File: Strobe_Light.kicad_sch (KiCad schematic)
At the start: 15 parts, among them J4 ErrorLightConn, Q1 NTR4003NT1G, Q2 VND5N07-E, U1 SI8261ABC-IS

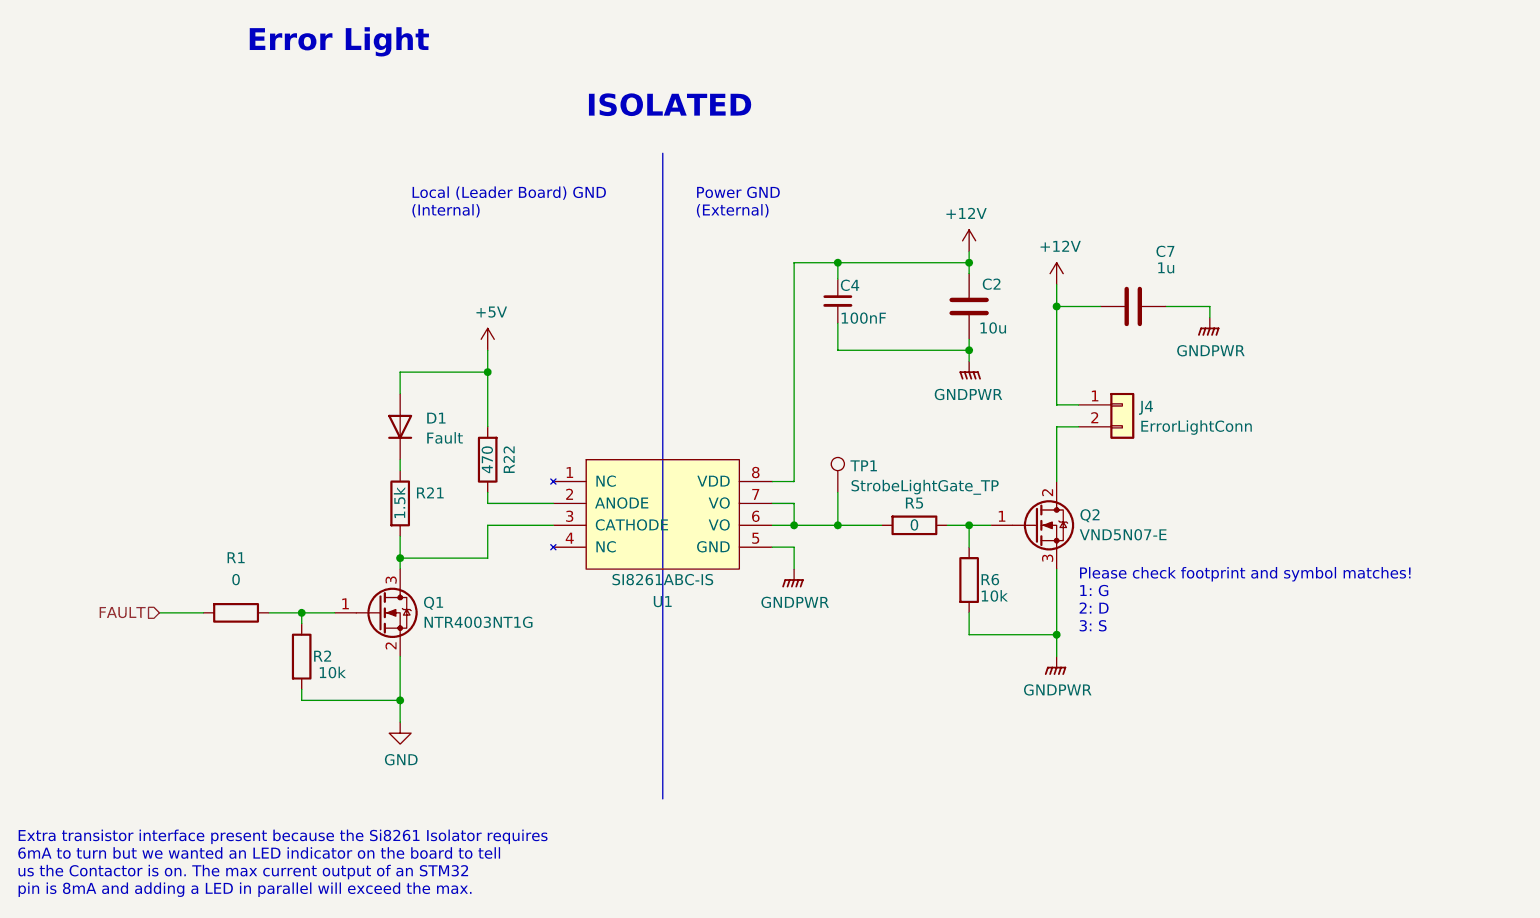
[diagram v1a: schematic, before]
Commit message: Finished comments for Strobe Light and started resolving them for Contactor
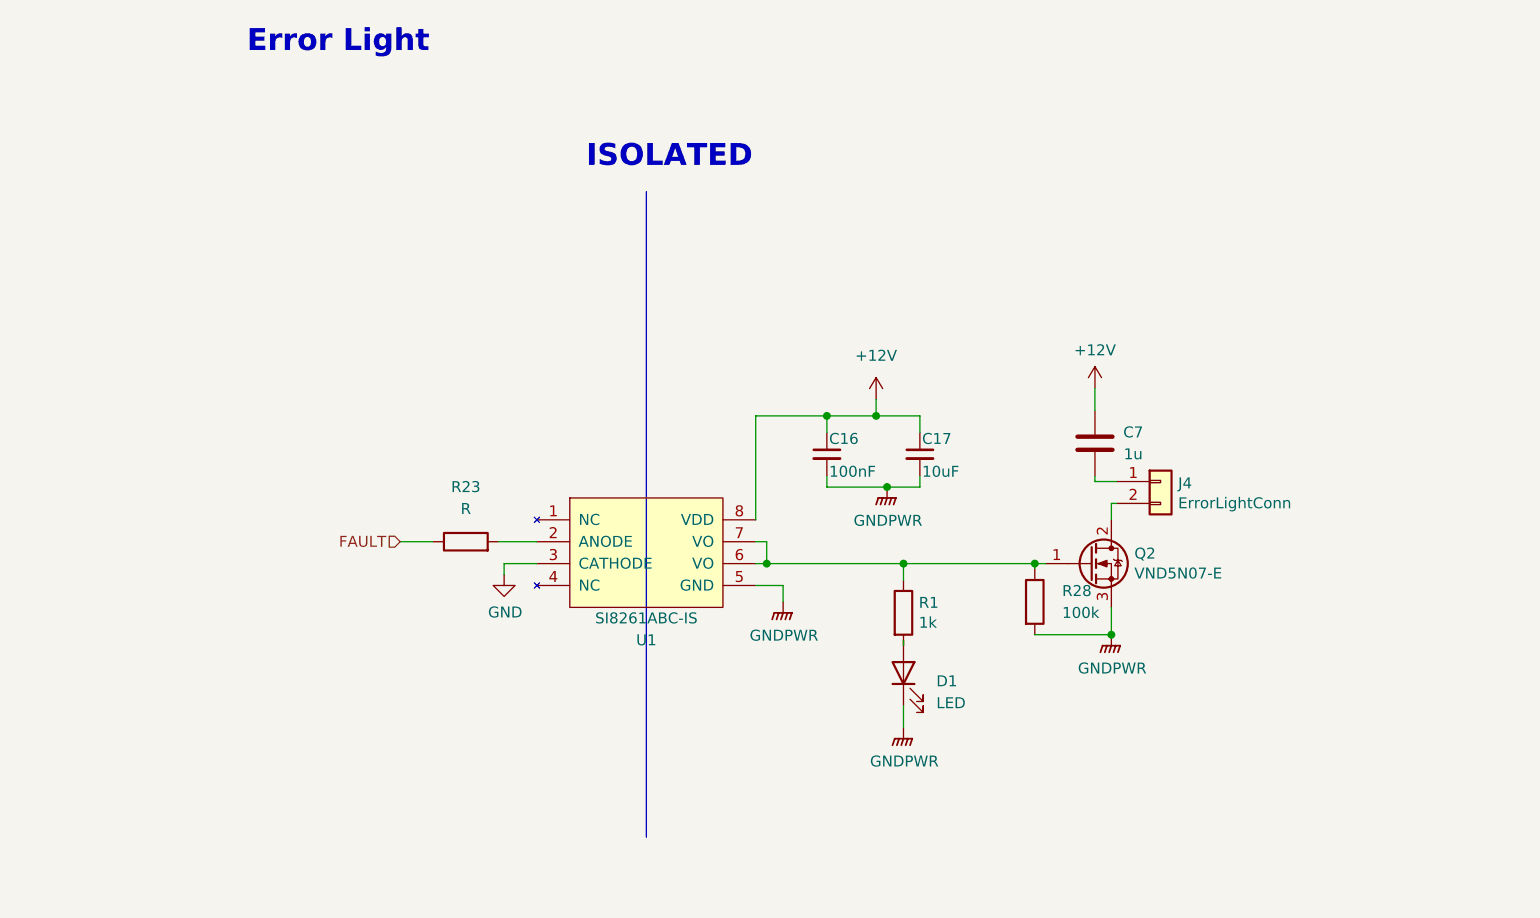
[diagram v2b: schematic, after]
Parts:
- removed C2: 10u, Capacitor_SMD:C_0805_2012Metric, symbol Device:C
- removed C4: 100nF, Capacitor_SMD:C_0805_2012Metric, symbol Device:C_Small
- removed D1: Fault, LED_SMD:LED_0805_2012Metric, symbol Device:D
- removed Q1: NTR4003NT1G, Package_TO_SOT_SMD:SOT-23, symbol Device:Q_NMOS_GSD
- removed R2, R6: 10k, Resistor_SMD:R_0805_2012Metric, symbol Device:R
- removed R21: 1.5k, Resistor_SMD:R_0805_2012Metric, symbol Device:R
- removed R22: 470, Resistor_SMD:R_0805_2012Metric, symbol Device:R
- removed R5: 0, Resistor_SMD:R_0805_2012Metric, symbol Device:R
- removed TP1: StrobeLightGate_TP, TestPoint:TestPoint_Keystone_5005-5009_Compact, symbol Connector:TestPoint
- added C16: 100nF, Capacitor_SMD:C_0805_2012Metric, symbol Device:C_Small
- added C17: 10uF, Capacitor_SMD:C_0805_2012Metric, symbol Device:C_Small
- added D1: LED, LED_SMD:LED_0805_2012Metric, symbol Device:LED
- added R23: R, symbol Device:R
- added R28: 100k, Resistor_SMD:R_0805_2012Metric, symbol Device:R
- R1: value 0 -> 1k; Mouser Part Number (none) -> 71-CRCW08051K00FKEAC; P/N CRCW08050000Z0EAC -> CRCW08051K00FKEAC
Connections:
- net +12V: now also C16.1, C17.1; no longer J4.1 (Pin_1)
- net FAULT: now also R23.1; no longer R1.2
- net GND: now also U1.3 (CATHODE)
- net GNDPWR: now also C16.2, C17.2, D1.1 (K), R28.2; no longer C7.2
- net at R1.1: now also Q2.1 (G), U1.6 (VO), U1.7 (VO), R28.1
- net at U1.2 (ANODE): now also R23.2
- new net: C7.2, J4.1 (Pin_1)
- new net: D1.2 (A), R1.2
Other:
- note removed: "Extra transistor interface present because the Si8261 Isolator requires 6mA to turn but we wanted an LED indicator on the board to tell us the Contactor is on. The max current output of an STM32 pin is 8mA and adding a LED in parallel will exceed the max."
- note removed: "Local (Leader Board) GND (Internal)"
- note removed: "Please check footprint and symbol matches! 1: G 2: D 3: S"
- note removed: "Power GND (External)"
